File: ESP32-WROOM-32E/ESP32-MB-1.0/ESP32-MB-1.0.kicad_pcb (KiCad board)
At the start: 2 copper layers, 125.6 x 91.4 mm, 52 parts, among them J1 Conn_01x19, J10 Conn_01x03_Pin, J11 Conn_01x03_Pin, J12 Conn_01x03_Pin, J13 Conn_01x03_Pin, J14 Conn_01x03_Pin, J15 Conn_01x03_Pin, J16 XT60-M, J2 Conn_01x19, J21 Conn_01x02_Pin, J22 XT60-M, J23 Conn_01x02_Pin, J24 Conn_01x02_Pin, J25 Conn_01x02_Pin, J26 Conn_01x02_Pin, J27 Conn_01x02_Pin, J28 Conn_01x02_Pin, J29 Conn_01x02_Pin, J3 Conn_01x19, J30 XT60-M, J31 Conn_01x02_Pin, J32 Conn_01x02_Pin, J33 Conn_01x11_Pin, J34 Conn_01x02_Pin, J35 Conn_01x02_Pin, J36 Conn_01x02_Pin, J37 Conn_01x02_Pin, J38 Conn_01x02_Pin, J39 Conn_01x02_Pin, J4 Conn_01x11_Pin, J5 Conn_01x11_Pin, J6 XT60-M, J7 Conn_01x19, J8 Conn_01x03_Pin, J9 Conn_01x03_Pin, U1 IRLB3813PBF, U2 IRLB3813PBF, U3 IRLB3813PBF, U4 IRLB3813PBF, U5 IRLB3813PBF, U6 IRLB3813PBF, U7 IRLB3813PBF, U8 IRLB3813PBF, U9 MCP2562-E-P

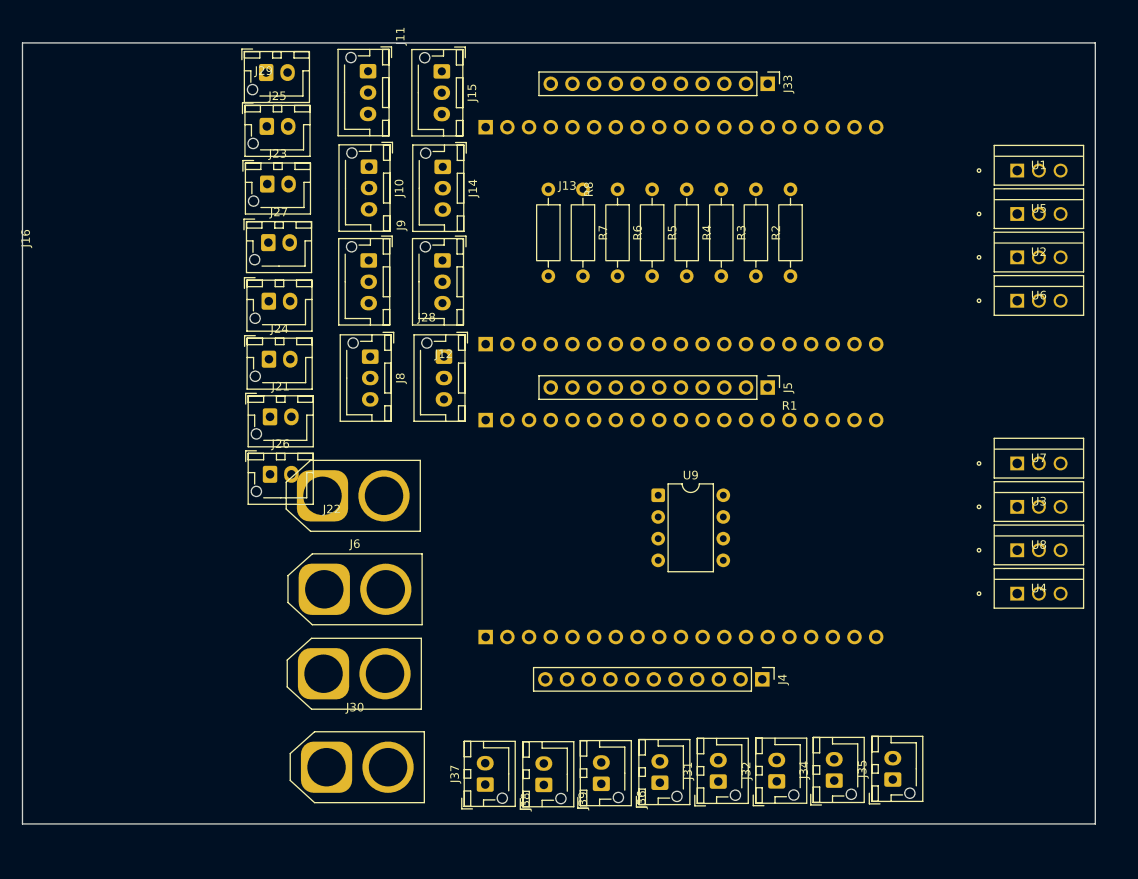
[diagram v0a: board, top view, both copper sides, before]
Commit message: 100になれなかったモタドラ4枚
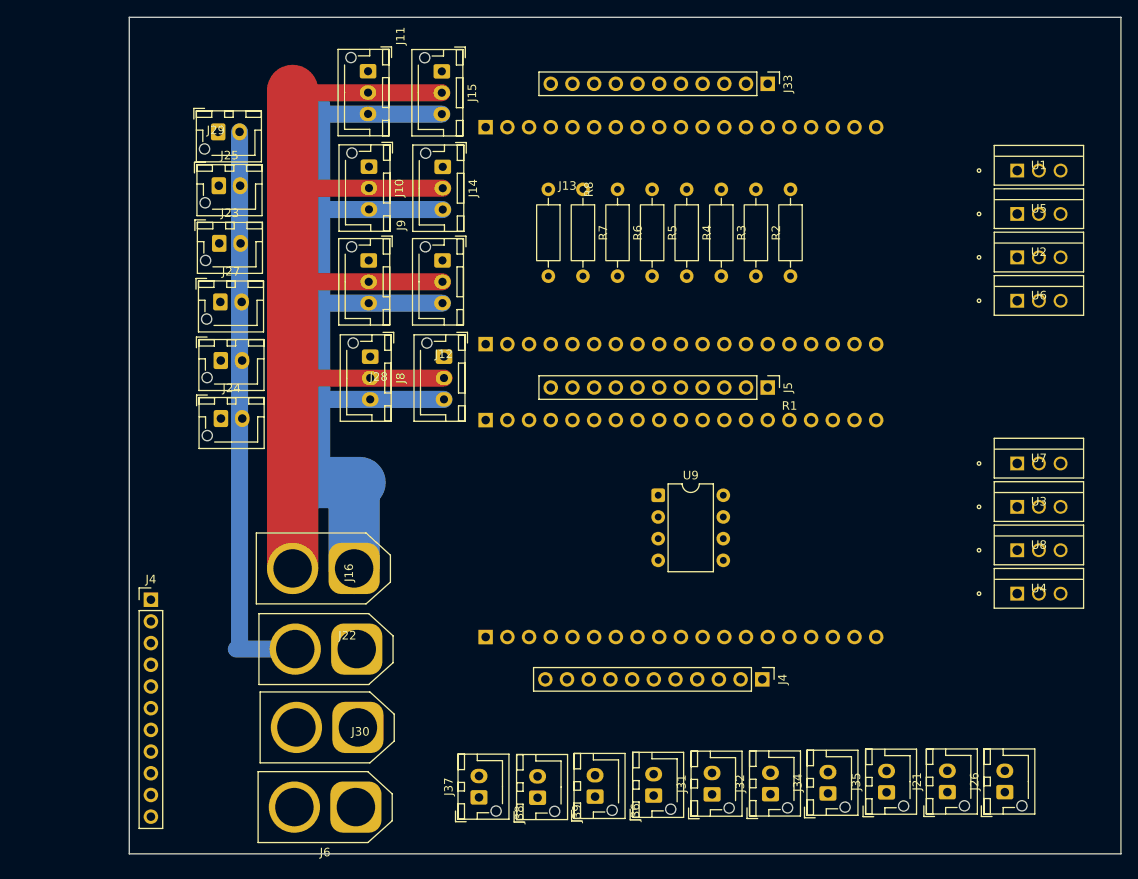
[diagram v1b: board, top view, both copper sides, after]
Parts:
- added J4: Conn_01x11_Pin, Connector_PinHeader_2.54mm:PinHeader_1x11_P2.54mm_Vertical, F.Cu at (134.0, 103.3)
- moved J26 93.7 mm to (234.0, 125.9), turned to 90 degrees
- moved J21 90.7 mm to (227.3, 125.9), turned to 90 degrees
- moved J6 25.8 mm to (158.0, 127.6), turned to 180 degrees
- moved J22 18.4 mm to (158.1, 109.1), turned to 180 degrees
- moved J16 12.8 mm to (157.8, 99.7), turned to 180 degrees
- moved J23 8.94 mm to (142.0, 61.6)
- moved J28 8.94 mm to (142.2, 75.3)
- moved J25 8.94 mm to (142.0, 54.9)
- moved J27 8.94 mm to (142.2, 68.5)
- moved J29 8.94 mm to (141.9, 48.6)
- moved J24 8.94 mm to (142.2, 82.1)
- moved J30 5.93 mm to (158.3, 118.3), turned to 180 degrees
- moved J31 1.67 mm to (199.7, 126.1)
- moved J32 1.67 mm to (206.6, 126.1)
- moved J34 1.67 mm to (213.3, 126.0)
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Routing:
- net +_servo: track 0.00 -> 128.9 mm
- net GND: track 0.00 -> 128.2 mm
- net 24V_IN: track 0.00 -> 67.6 mm
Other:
- board size 125.6 x 91.4 mm -> 116.1 x 97.9 mm
